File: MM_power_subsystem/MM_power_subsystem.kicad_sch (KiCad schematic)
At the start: 21 parts, among them J1 Conn_01x02_Socket, J2 Conn_02x16_Top_Bottom, Q1 2N2219, SW1 SW_SPST, U2 AMS1117-3.3, U3 MCP73831-2-OT, U4 MT3608

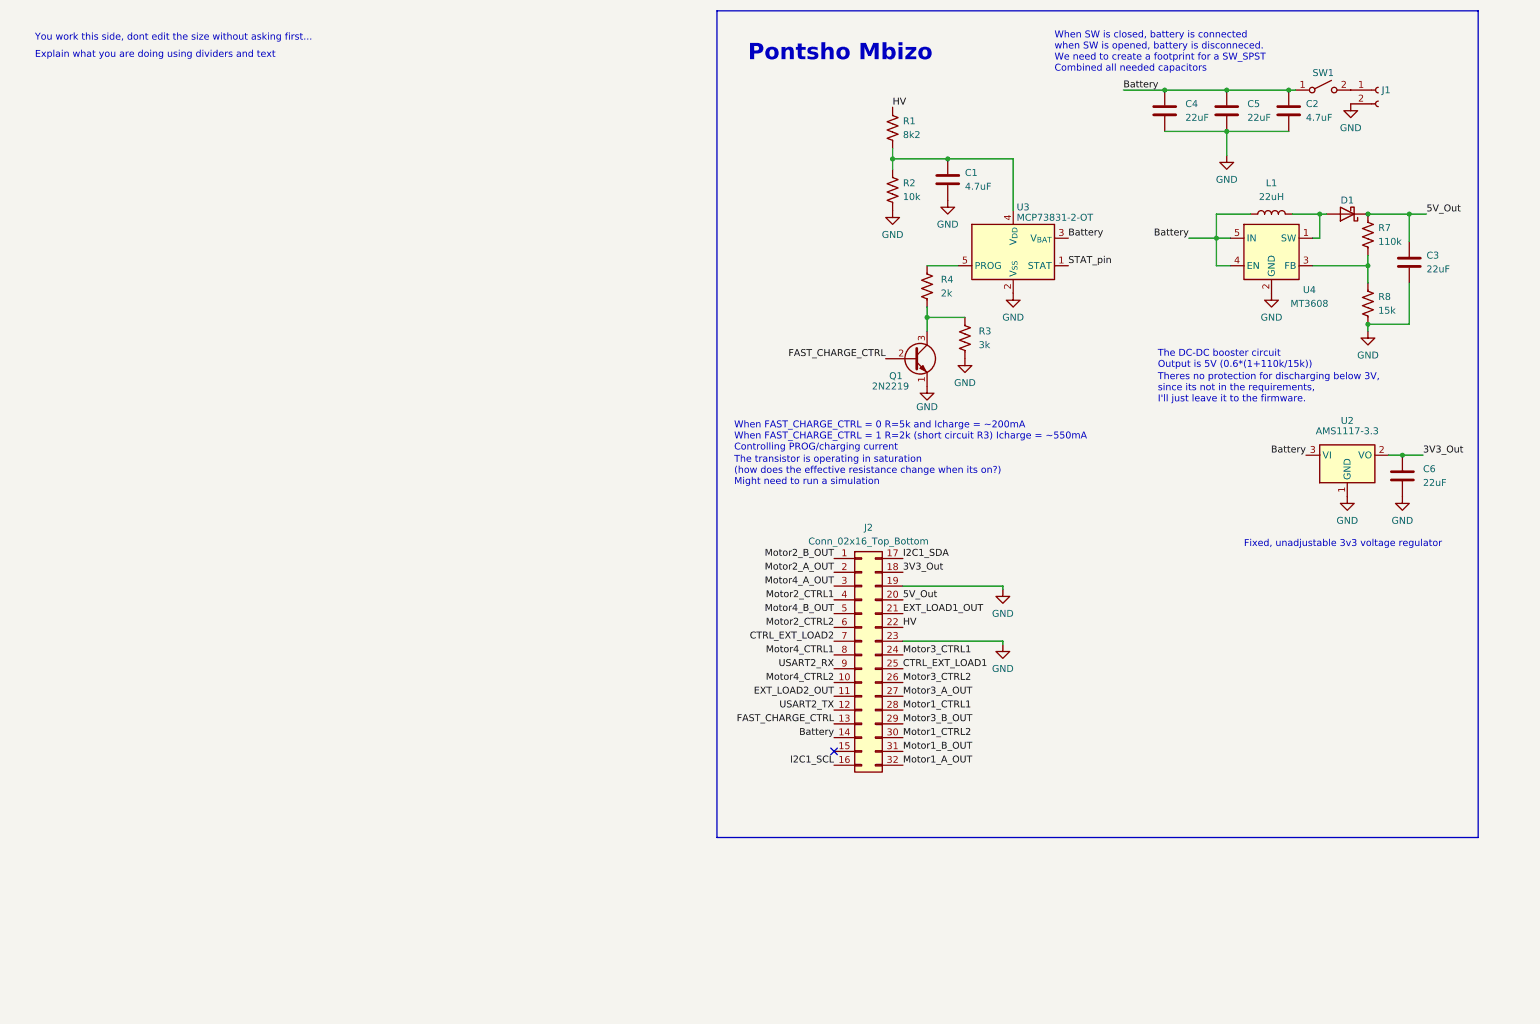
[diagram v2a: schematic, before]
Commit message: finalized part 2 schematic
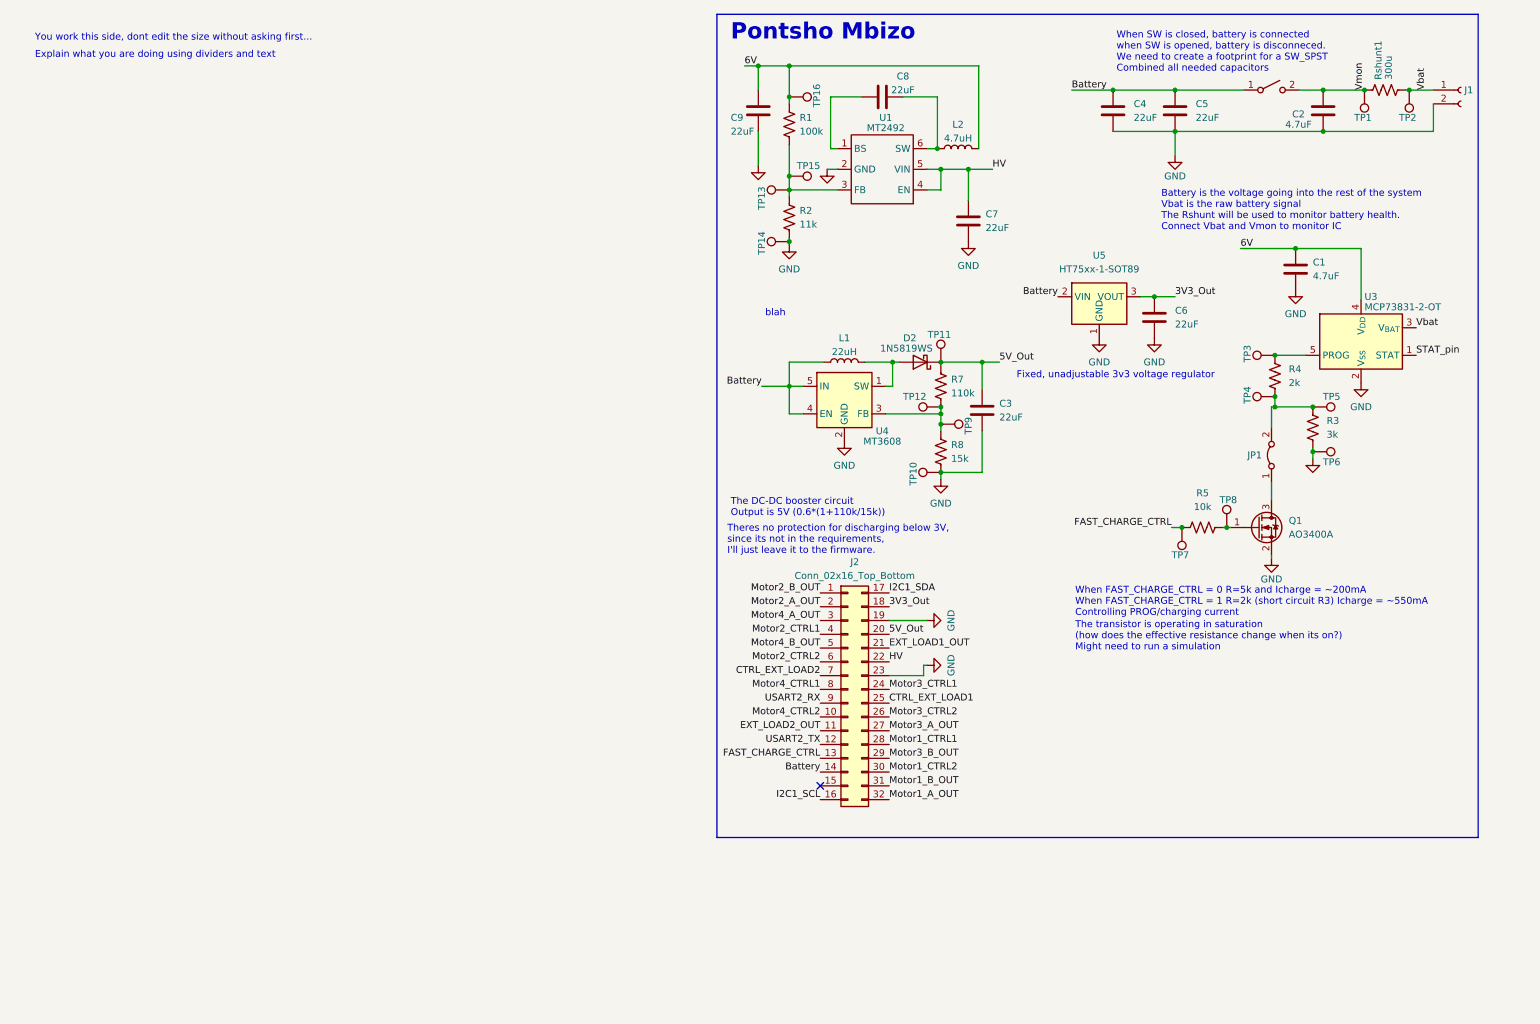
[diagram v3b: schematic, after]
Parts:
- removed D1: 1N5819, Diode_THT:D_DO-41_SOD81_P10.16mm_Horizontal, symbol Diode:1N5819
- removed Q1: 2N2219, Package_TO_SOT_THT:TO-39-3, symbol Transistor_BJT:2N2219
- removed U2: AMS1117-3.3, Package_TO_SOT_SMD:SOT-223-3_TabPin2, symbol Regulator_Linear:AMS1117-3.3
- added C7, C8, C9: 22uF, symbol Device:C
- added D2: 1N5819WS, Diode_SMD:D_SOD-323, symbol Diode:1N5819WS
- added JP1: Jumper_2_Bridged, symbol Jumper:Jumper_2_Bridged
- added L2: 4.7uH, symbol Device:L
- added Q1: AO3400A, Package_TO_SOT_SMD:SOT-23, symbol Transistor_FET:AO3400A
- added R5: 10k, symbol Device:R_US
- added Rshunt1: 300u, symbol Device:R_US
- added TP1, TP10, TP11, TP12, TP13, TP14, TP15, TP16, TP2, TP3, TP4, TP5, TP6, TP7, TP8, TP9: TestPoint, symbol Connector:TestPoint
- added U1: MT2492, symbol MM_library:MT2492
- added U5: HT75xx-1-SOT89, Package_TO_SOT_SMD:SOT-89-3, symbol Regulator_Linear:HT75xx-1-SOT89
- R1: value 8k2 -> 100k
- R2: value 10k -> 11k
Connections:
- net 3V3_Out: now also U5.3 (VOUT)
- net 5V_Out: now also D2.1 (K), TP11.1
- net Battery: now also U5.2 (VIN); no longer C2.1, U3.3 (V_{BAT})
- net FAST_CHARGE_CTRL: now also R5.1, TP7.1
- net GND: now also C7.2, C9.2, Q1.2 (S), TP10.1, TP14.1, TP6.1, U1.2 (GND), U5.1 (GND)
- net HV: now also C7.1, U1.4 (EN), U1.5 (VIN); no longer R1.1
- net at L1.2, U4.1 (SW): now also D2.2 (A)
- net at R7.2, R8.1, U4.3 (FB): now also TP12.1, TP9.1
- net at R4.1, U3.5 (PROG): now also TP3.1
- net at R3.1, R4.2: now also JP1.2 (B), TP4.1, TP5.1
- net at R1.2, R2.1: now also TP13.1, TP15.1, U1.3 (FB); no longer C1.1, U3.4 (V_{DD})
- net Vbat: now reaches J1.1 (Pin_1)
- net Vbat: now also U3.3 (V_{BAT}), Rshunt1.2, TP2.1; no longer SW1.2 (B)
- new net: JP1.1 (A), Q1.3 (D)
- new net: C8.2, L2.1, U1.6 (SW)
- new net: Q1.1 (G), R5.2, TP8.1
- new net: C8.1, U1.1 (BS)
- new net 6V: C1.1, C9.1, L2.2, R1.1, TP16.1, U3.4 (V_{DD})
- new net Vmon: C2.1, Rshunt1.1, SW1.2 (B), TP1.1
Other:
- note added: "Battery is the voltage going into the rest of the system Vbat is the raw battery signal The Rshunt will be used to monitor battery health. Connect Vbat and Vmon to monitor IC"
- note added: "blah"
- moved on the sheet: C1, C3, C4, C5, C6, J1, J2, L1, R3, R4, R7, R8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
